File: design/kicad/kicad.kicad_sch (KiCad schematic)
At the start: 18 parts, among them J1 Raspberry_Pi_4, J2 Conn_01x05, J3 Conn_01x05, J4 Conn_01x08, Q1 AO3401A, Q2 AO3401A, Q3 AO3401A, SW1 SW_Shutdown

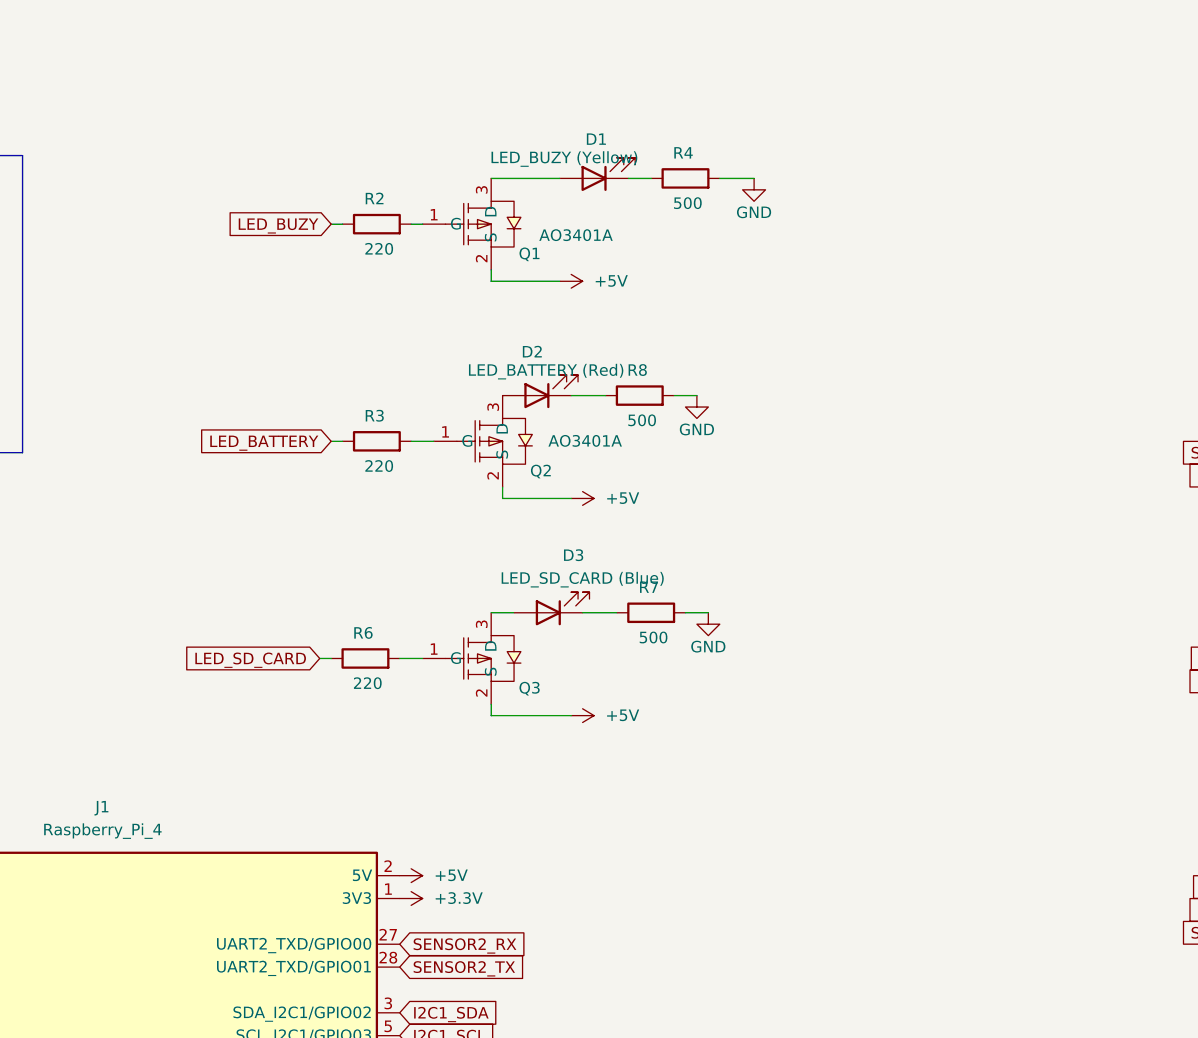
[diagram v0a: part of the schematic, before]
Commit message: prod update
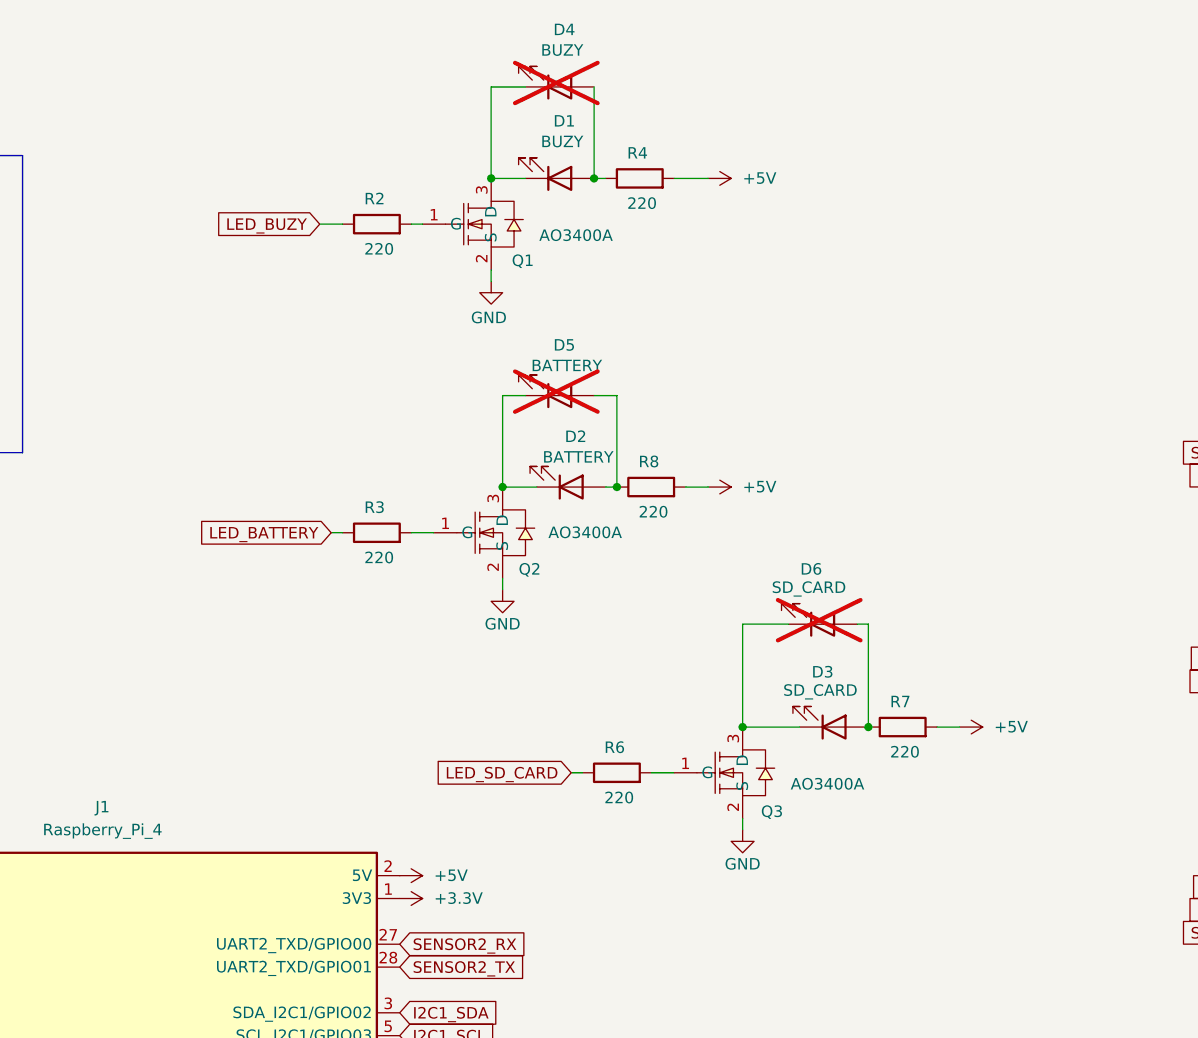
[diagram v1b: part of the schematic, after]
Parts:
- added D4: BUZY, easyeda2kicad:LED-TH_BD3.9-P2.54-FD, symbol Device:LED
- added D5: BATTERY, easyeda2kicad:LED-TH_BD3.9-P2.54-FD, symbol Device:LED
- added D6: SD_CARD, easyeda2kicad:LED-TH_BD3.9-P2.54-FD, symbol Device:LED
- D1: value LED_BUZY (Yellow) -> BUZY; footprint LED_THT:LED_D3.0mm_Horizontal_O1.27mm_Z2.0mm -> easyeda2kicad:LED-SMD_L1.7-W0.6-RD-custom; LCSC Part C330775 -> C133119
- D2: value LED_BATTERY (Red) -> BATTERY; footprint LED_THT:LED_D3.0mm_Horizontal_O1.27mm_Z2.0mm -> easyeda2kicad:LED-SMD_L1.7-W0.6-RD-custom; LCSC Part C330774 -> C125114
- D3: value LED_SD_CARD (Blue) -> SD_CARD; footprint LED_THT:LED_D3.0mm_Horizontal_O1.27mm_Z2.0mm -> easyeda2kicad:LED-SMD_L1.7-W0.6-RD-custom; LCSC Part C330750 -> C125115
- J1: footprint Connector_PinSocket_2.54mm:PinSocket_2x20_P2.54mm_Vertical -> easyeda2kicad:HDR-TH_40P-P2.54-V-F-R2-C20-S2.54-2-reveresed
- J2, J3: footprint Connector_JST:JST_PH_S5B-PH-K_1x05_P2.00mm_Horizontal -> easyeda2kicad:CONN-TH_WAFER-HA254WZ-5A
- Q1, Q2, Q3: value AO3401A -> AO3400A; footprint Package_TO_SOT_SMD:SOT-23W -> easyeda2kicad:SOT-23-3_L2.9-W1.3-P1.90-LS2.4-BR; symbol easyeda2kicad:AO3401A -> easyeda2kicad:AO3400A; LCSC Part C15127 -> C20917
- R4, R7, R8: value 500 -> 220; LCSC Part C17734 -> C17557
- SW1: footprint Button_Switch_THT:SW_Tactile_SPST_Angled_PTS645Vx83-2LFS -> easyeda2kicad:SW-TH_TK-6580B-2; LCSC Part C318869 -> C2689830
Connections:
- net +5V: now also R4.2, R7.2, R8.2; no longer Q1.2 (S), Q2.2 (S), Q3.2 (S)
- net GND: now also Q1.2 (S), Q2.2 (S), Q3.2 (S); no longer R4.2, R7.2, R8.2
- net at Q2.3 (D): now also D2.1 (K), D5.1 (K); no longer D2.2 (A)
- net at D1.1 (K): now also Q1.3 (D), D4.1 (K); no longer R4.1
- net at D1.2 (A): now also R4.1, D4.2 (A); no longer Q1.3 (D)
- net at R7.1: now also D3.2 (A), D6.2 (A); no longer D3.1 (K)
- net at R8.1: now also D2.2 (A), D5.2 (A); no longer D2.1 (K)
- net at Q3.3 (D): now also D3.1 (K), D6.1 (K); no longer D3.2 (A)
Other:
- moved on the sheet: D1, D2, D3, R3, R4, R6, R7, R8
